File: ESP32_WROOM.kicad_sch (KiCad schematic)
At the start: 11 parts, among them J7 Programming Socket, Q1 NPN, Q2 NPN, SW1 EN, SW2 EN, U11 NTS0104GU12_115, U6 ESP32-WROOM-32E

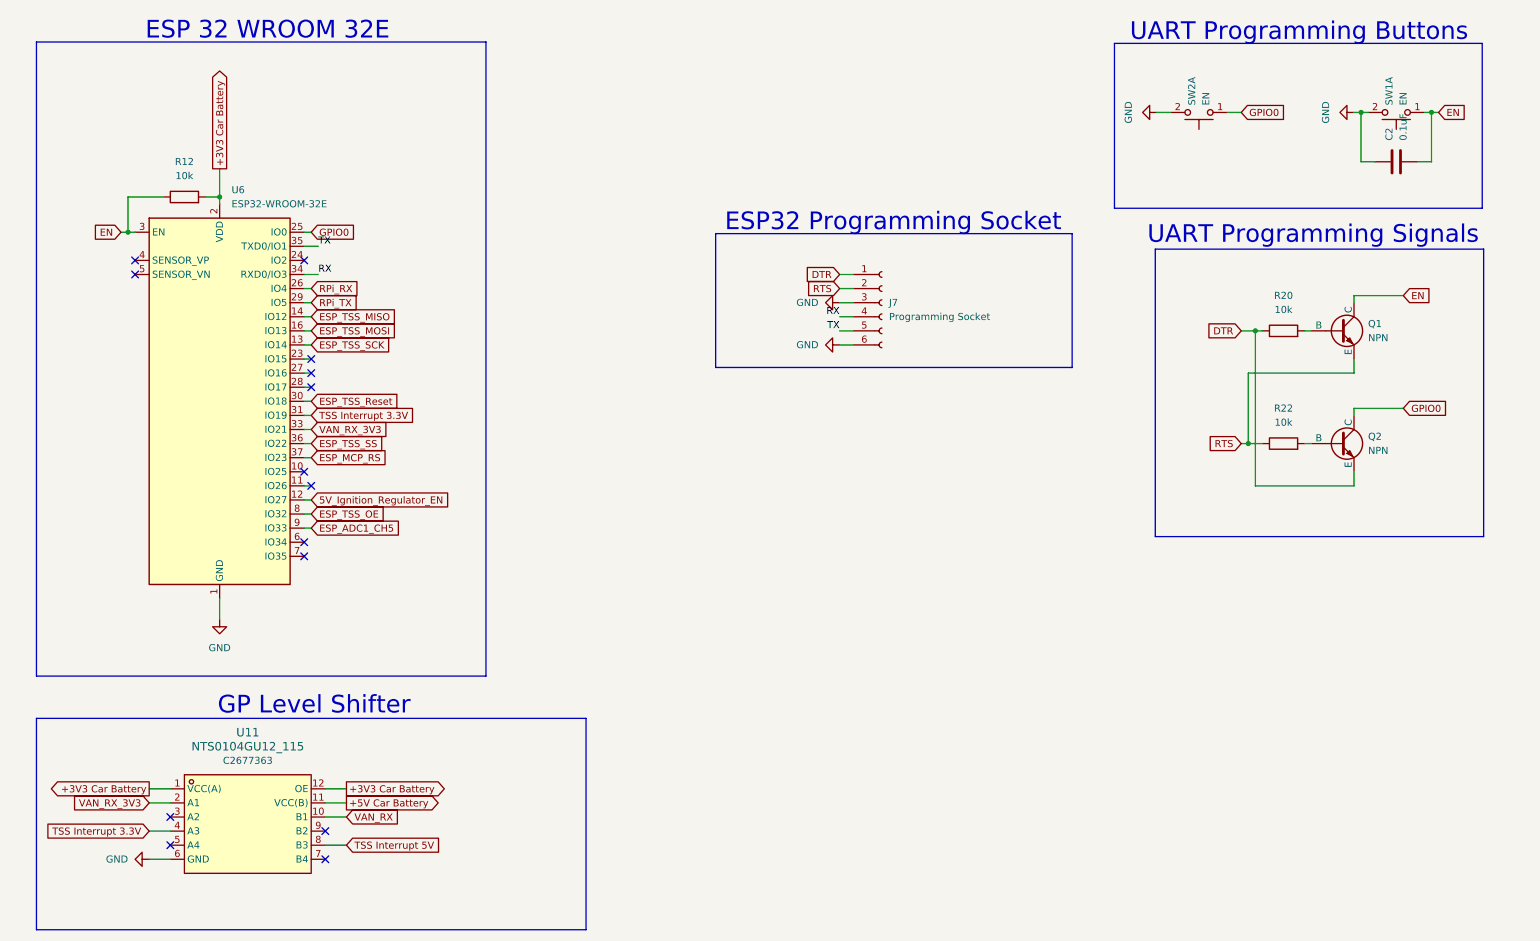
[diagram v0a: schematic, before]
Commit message: 2 layer PCB
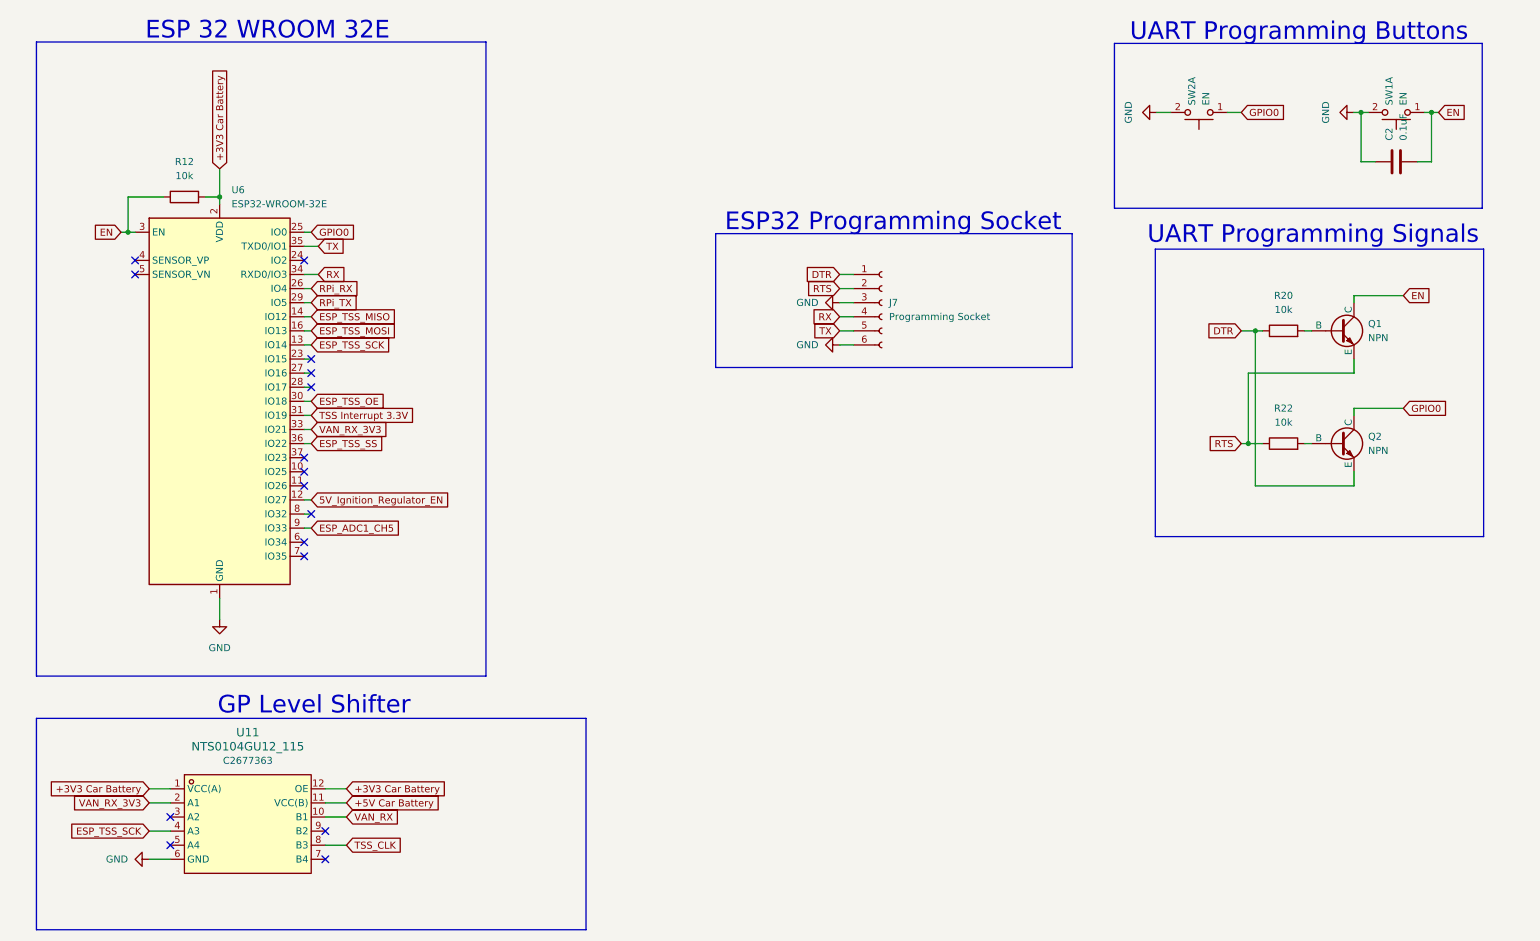
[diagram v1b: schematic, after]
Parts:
- U6: footprint RF_Module:ESP32-WROOM-32D -> intoftainment:esp32_altered
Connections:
- net ESP_TSS_Reset is gone; now on net ESP_TSS_OE: U6.30 (IO18)
- net ESP_TSS_OE: no longer U6.8 (IO32)
- net ESP_TSS_SCK: now also U11.4 (A3)
- net TSS Interrupt 3.3V: no longer U11.4 (A3)
- net ESP_MCP_RS: no longer names the net of U6.37 (IO23)
- net TSS Interrupt 5V renamed TSS_CLK
- no-connect marks 14 -> 16
